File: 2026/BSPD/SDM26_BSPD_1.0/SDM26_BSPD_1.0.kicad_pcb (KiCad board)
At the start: 4 copper layers, 90 x 41 mm, 71 parts, among them IC1 LM2901BIRTER, IC2 LM2901BIRTER, IC3 SN74HC08PWR, IC4 SN74HC32PWR, IC5 L7805ACD2T-TR, J1 776280-1, Q1 2N7002,215, U1 TPS2116DRL

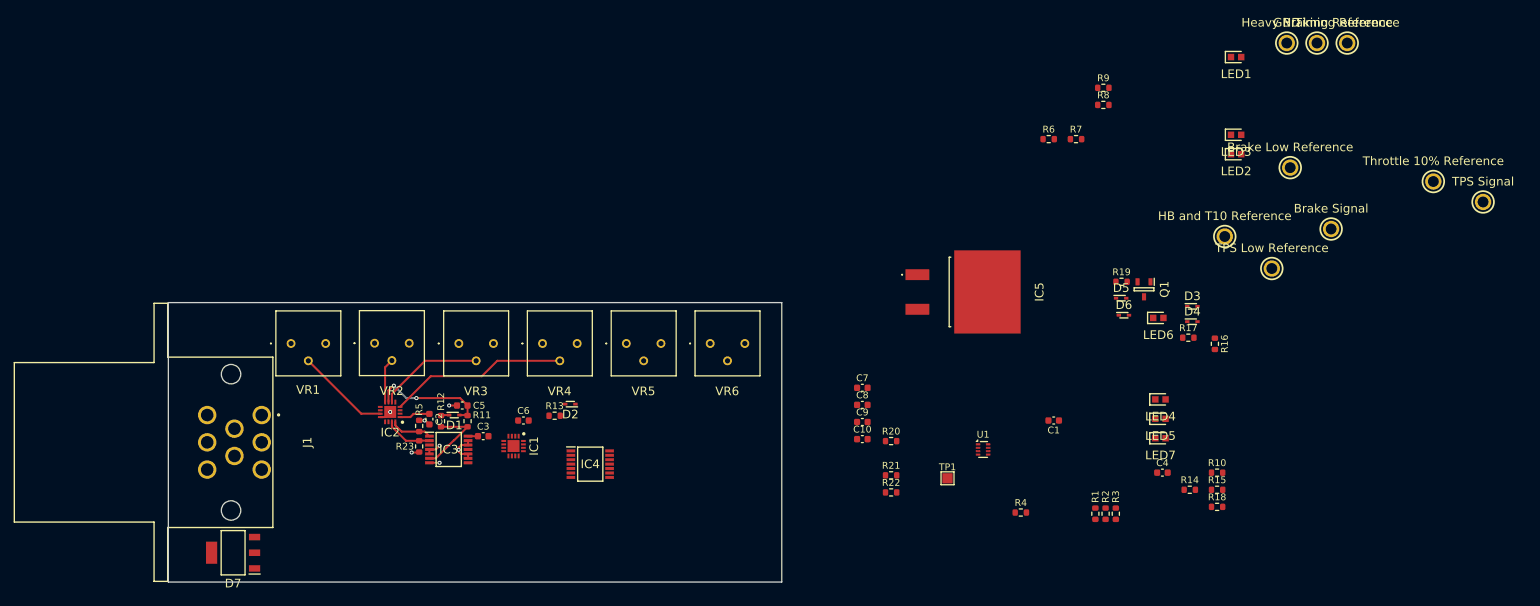
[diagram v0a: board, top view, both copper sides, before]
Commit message: Minor fixes
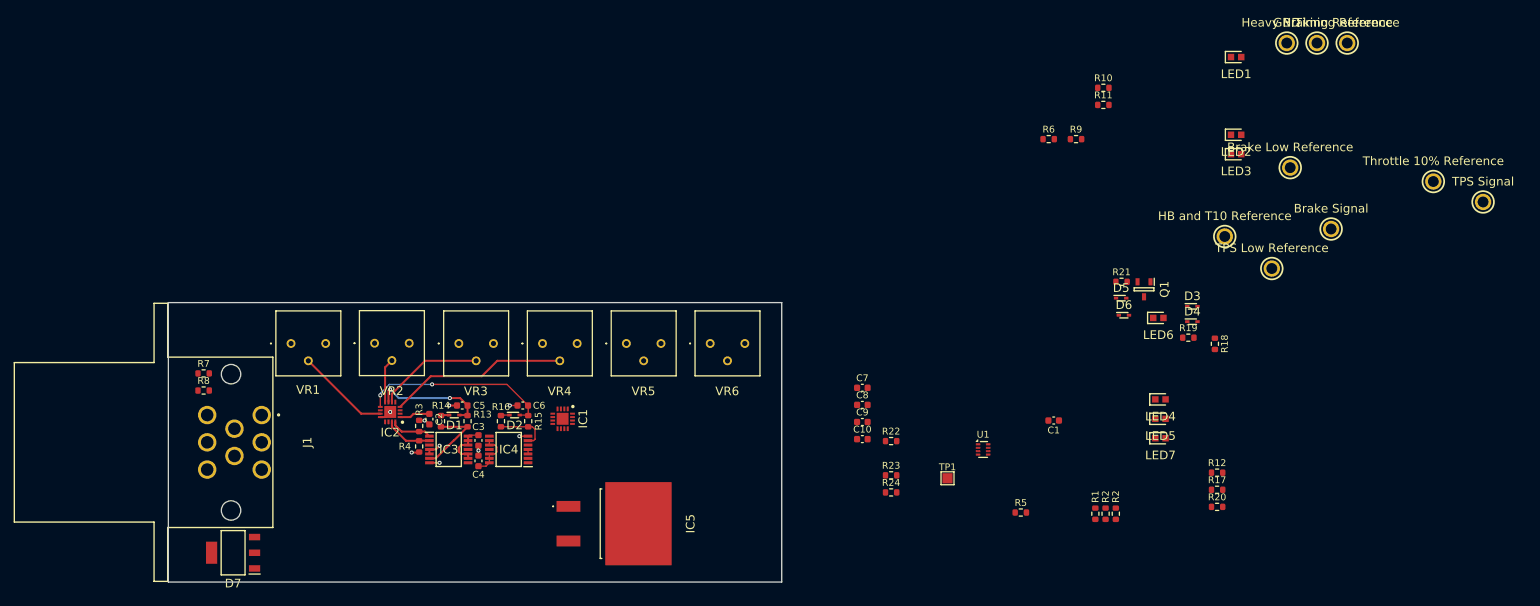
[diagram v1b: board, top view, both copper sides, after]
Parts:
- added R7: 10k, Resistor_SMD:R_0603_1608Metric, F.Cu at (55.2, 110.4)
- added R8: 10k, Resistor_SMD:R_0603_1608Metric, F.Cu at (55.2, 112.9)
- moved R16 101.6 mm to (98.8, 117.4), turned to 90 degrees
- moved C4 100.4 mm to (95.5, 123.2), turned to 90 degrees
- moved IC5 61.5 mm to (115.6, 132.4)
- moved IC4 12.2 mm to (99.9, 121.5), turned to 180 degrees
- moved D2 8.33 mm to (100.8, 116.5), turned to 0 degrees
- moved IC1 8.24 mm to (107.8, 117.0)
- moved R15 3.96 mm to (102.8, 117.4), turned to 90 degrees
- moved C6 2.20 mm to (102.0, 115.1), turned to 180 degrees
- moved C3 0.94 mm to (95.5, 120.2), turned to -90 degrees
- renumbered LED3 to LED2, LED2 to LED3, R9 to R10, R8 to R11, R10 to R12, R11 to R13, R12 to R14, R13 to R15, R14 to R16, R15 to R17, R16 to R18, R17 to R19, R3 to R2, R18 to R20, R19 to R21, R20 to R22, R21 to R23, R22 to R24, R5 to R3, R23 to R4, R4 to R5, R7 to R9, RED_TP4 to RED_TP2, RED_TP2 to RED_TP3, RED_TP3 to RED_TP4
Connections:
- C3 pad 1: Net-(IC3-VCC) -> Net-(IC3-3A)
- C4 pad 1: Net-(IC4-VCC) -> Net-(IC4-3A)
- IC3 pad 10: GND -> Net-(IC3-3A)
- IC3 pad 12: GND -> Net-(IC3-3A)
- IC3 pad 13: GND -> Net-(IC3-3A)
- IC3 pad 14: Net-(IC3-VCC) -> Net-(IC3-3A)
- IC3 pad 9: GND -> Net-(IC3-3A)
- IC4 pad 10: GND -> Net-(IC4-3A)
- IC4 pad 12: GND -> Net-(IC4-3A)
- IC4 pad 13: GND -> Net-(IC4-3A)
- IC4 pad 14: Net-(IC4-VCC) -> Net-(IC4-3A)
- IC4 pad 9: GND -> Net-(IC4-3A)
- RED_TP5 pad 1: Net-(VR5-Wiper) -> /TPS_LOW_REF
- RED_TP6 pad 1: Net-(VR6-Wiper) -> /BRAKE_LOW_REF
- VR5 pad 2: Net-(VR5-Wiper) -> /TPS_LOW_REF
- VR6 pad 2: Net-(VR6-Wiper) -> /BRAKE_LOW_REF
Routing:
- net /BL+TL+(HB*T10)_FAULT: track 0.00 -> 28.2 mm, vias 0 -> 2
- net Net-(IC4-2Y): track 0.00 -> 7.71 mm
- net Net-(IC3-3A): track 0.00 -> 7.14 mm
- net Net-(IC4-3A): track 0.00 -> 6.91 mm
- net GND: track 11.7 -> 9.19 mm, vias 5 -> 6
- net +5V: track 2.88 -> 4.33 mm, vias 2 -> 3
- net Net-(IC3-VCC): track 1.45 -> 0.00 mm
- net Net-(D2-K): track 0.00 -> 1.28 mm
- net /BL+TL_FAULT: track 0.00 -> 0.65 mm
